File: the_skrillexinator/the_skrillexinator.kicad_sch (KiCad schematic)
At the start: 0 parts

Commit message: add shit
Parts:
- added J1, J2: Conn_01x03, symbol Connector_Generic:Conn_01x03
- added U1: ESP32-WROOM-32, RF_Module:ESP32-WROOM-32, symbol RF_Module:ESP32-WROOM-32
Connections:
- new net: J2.2 (Pin_2), U1.36 (IO22)
- new net +3.3V: J2.3 (Pin_3), U1.2 (VDD)
- new net GND: J2.1 (Pin_1), U1.1 (GND), U1.15 (GND), U1.38 (GND), U1.39 (GND)

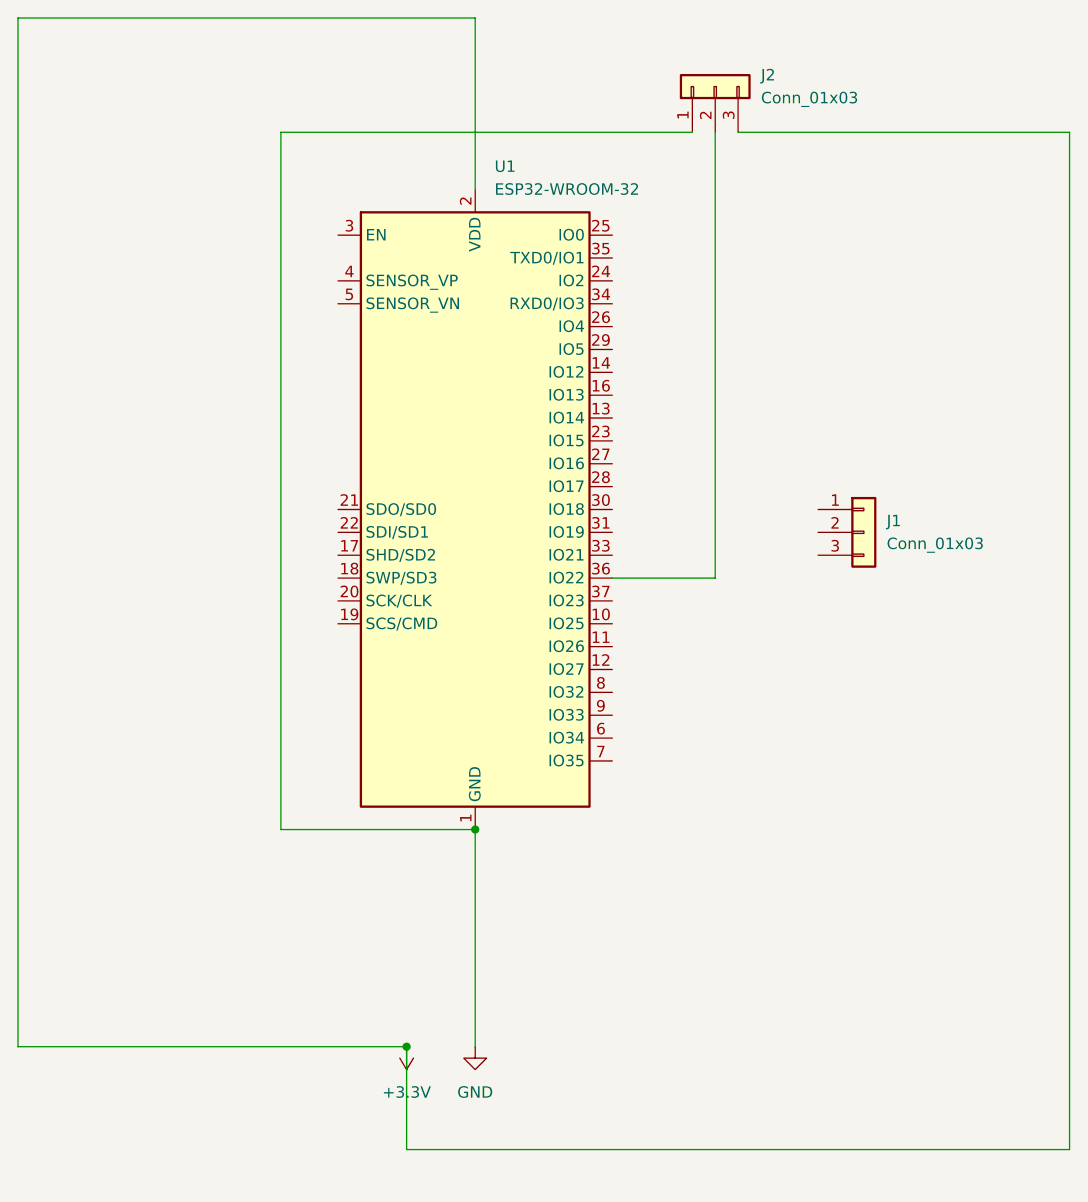
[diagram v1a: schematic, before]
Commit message: add resistor shit
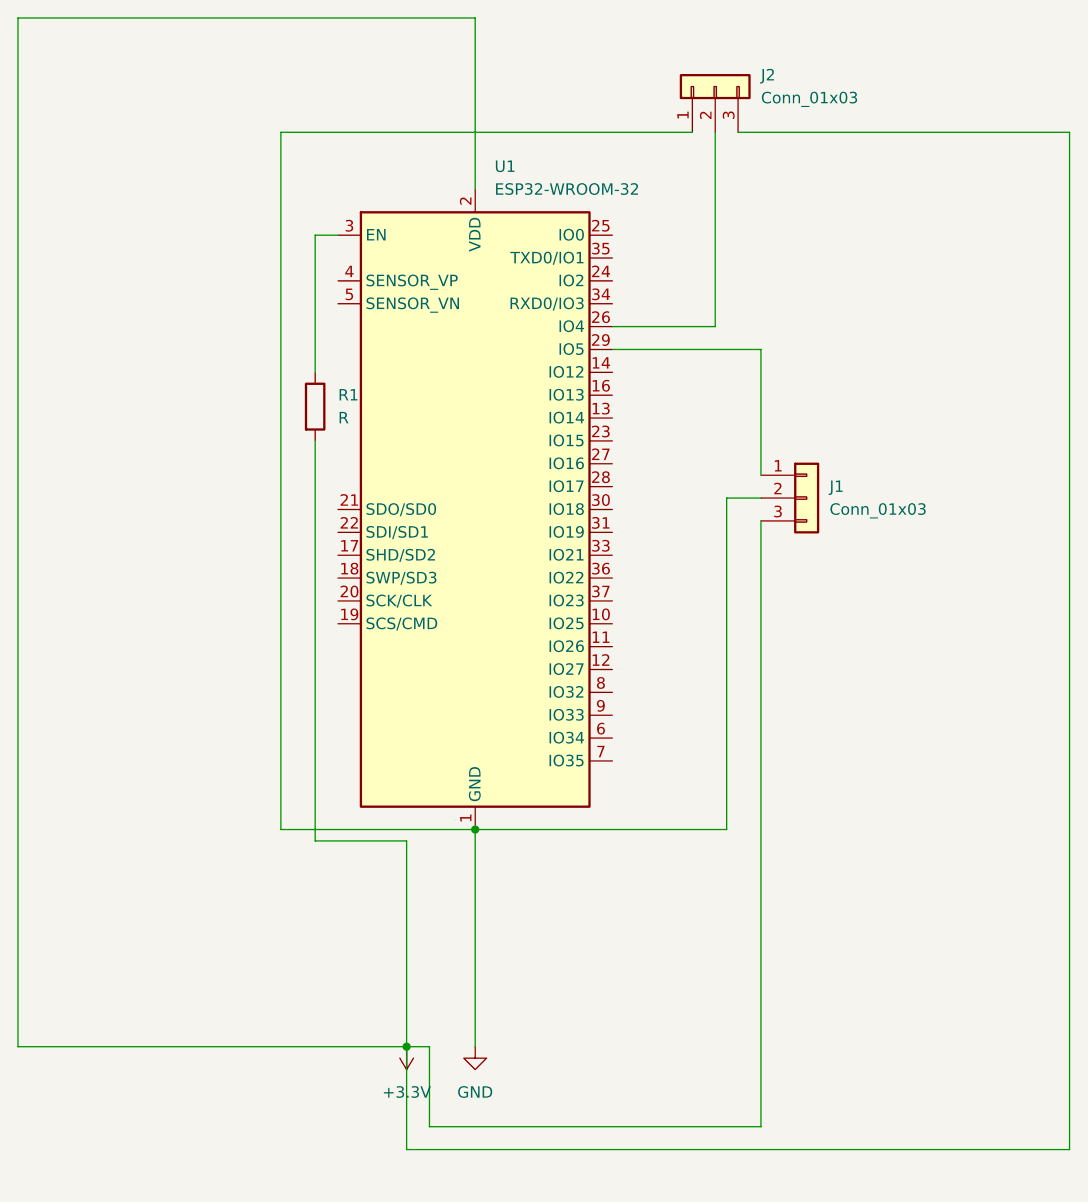
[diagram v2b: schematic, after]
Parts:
- added R1: R, symbol Device:R
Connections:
- net +3.3V: now also J1.3 (Pin_3), R1.2
- net GND: now also J1.2 (Pin_2)
- net at U1.26 (IO4): now also J2.2 (Pin_2)
- net at U1.29 (IO5): now also J1.1 (Pin_1)
- net at U1.3 (EN): now also R1.1
- net at U1.36 (IO22): no longer J2.2 (Pin_2)
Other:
- moved on the sheet: J1
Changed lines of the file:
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@@
+	(wire
+		(pts
+			(xy 181.61 76.2) (xy 181.61 62.23)
+		)
+		(stroke
+			(width 0)
+			(type default)
+		)
+	)
 	(wire
 		(pts
@@
 	(wire
 		(pts
+			(xy 132.08 116.84) (xy 142.24 116.84)
+		)
+		(stroke
+			(width 0)
+			(type default)
+		)
+	)
+	(wire
+		(pts
+			(xy 176.53 59.69) (xy 165.1 59.69)
+		)
+		(stroke
+			(width 0)
+			(type default)
+		)
+	)
+	(wire
+		(pts
+			(xy 132.08 64.77) (xy 132.08 49.53)
+		)
+		(stroke
+			(width 0)
+			(type default)
+		)
+	)
+	(wire
+		(pts
 			(xy 149.86 25.4) (xy 99.06 25.4)
 		)
@@
 	(wire
 		(pts
+			(xy 144.78 148.59) (xy 144.78 139.7)
+		)
+		(stroke
+			(width 0)
+			(type default)
+		)
+	)
+	(wire
+		(pts
+			(xy 181.61 78.74) (xy 177.8 78.74)
+		)
+		(stroke
+			(width 0)
+			(type default)
+		)
+	)
+	(wire
+		(pts
 			(xy 215.9 38.1) (xy 215.9 151.13)
 		)
@@
 	(wire
 		(pts
+			(xy 142.24 116.84) (xy 142.24 139.7)
+		)
+		(stroke
+			(width 0)
+			(type default)
+		)
+	)
+	(wire
+		(pts
 			(xy 128.27 115.57) (xy 149.86 115.57)
 		)
@@
 	(wire
 		(pts
-			(xy 165.1 87.63) (xy 176.53 87.63)
+			(xy 181.61 62.23) (xy 165.1 62.23)
+		)
+		(stroke
+			(width 0)
+			(type default)
+		)
+	)
+	(wire
+		(pts
+			(xy 176.53 38.1) (xy 176.53 59.69)
 		)
 		(stroke
@@
 	(wire
 		(pts
-			(xy 176.53 87.63) (xy 176.53 38.1)
+			(xy 132.08 49.53) (xy 134.62 49.53)
+		)
+		(stroke
+			(width 0)
+			(type default)
+		)
+	)
+	(wire
+		(pts
+			(xy 132.08 72.39) (xy 132.08 116.84)
 		)
 		(stroke
@@
 	(wire
 		(pts
+			(xy 177.8 78.74) (xy 177.8 115.57)
+		)
+		(stroke
+			(width 0)
+			(type default)
+		)
+	)
+	(wire
+		(pts
 			(xy 149.86 44.45) (xy 149.86 25.4)
 		)
@@
 	(wire
 		(pts
+			(xy 177.8 115.57) (xy 149.86 115.57)
+		)
+		(stroke
+			(width 0)
+			(type default)
+		)
+	)
+	(wire
+		(pts
+			(xy 181.61 148.59) (xy 144.78 148.59)
+		)
+		(stroke
+			(width 0)
+			(type default)
+		)
+	)
+	(wire
+		(pts
 			(xy 99.06 139.7) (xy 142.24 139.7)
 		)
@@
 	(wire
 		(pts
+			(xy 181.61 81.28) (xy 181.61 148.59)
+		)
+		(stroke
+			(width 0)
+			(type default)
+		)
+	)
+	(wire
+		(pts
+			(xy 144.78 139.7) (xy 142.24 139.7)
+		)
+		(stroke
+			(width 0)
+			(type default)
+		)
+	)
+	(wire
+		(pts
 			(xy 215.9 151.13) (xy 142.24 151.13)
 		)
@@
 			(width 0)
 			(type default)
+		)
+	)
+	(symbol
+		(lib_id "Device:R")
+		(at 132.08 68.58 0)
+		(unit 1)
+		(body_style 1)
+		(exclude_from_sim no)
+		(in_bom yes)
+		(on_board yes)
+		(in_pos_files yes)
+		(dnp no)
+		(fields_autoplaced yes)
+		(property "Reference" "R1"
+			(at 134.62 67.3099 0)
+			(show_name no)
+			(do_not_autoplace no)
+			(effects
+				(font
+					(size 1.27 1.27)
+				)
+				(justify left)
+			)
+		)
+		(property "Value" "R"
+			(at 134.62 69.8499 0)
+			(show_name no)
+			(do_not_autoplace no)
+			(effects
+				(font
+					(size 1.27 1.27)
+				)
+				(justify left)
+			)
+		)
+		(property "Footprint" ""
+			(at 130.302 68.58 90)
+			(hide yes)
+			(show_name no)
+			(do_not_autoplace no)
+			(effects
+				(font
+					(size 1.27 1.27)
+				)
+			)
+		)
+		(property "Datasheet" ""
+			(at 132.08 68.58 0)
+			(hide yes)
+			(show_name no)
+			(do_not_autoplace no)
+			(effects
+				(font
+					(size 1.27 1.27)
+				)
+			)
+		)
+		(property "Description" "Resistor"
+			(at 132.08 68.58 0)
+			(hide yes)
+			(show_name no)
+			(do_not_autoplace no)
+			(effects
+				(font
+					(size 1.27 1.27)
+				)
+			)
+		)
+		(pin "1"
+		)
+		(pin "2"
+		)
+		(instances
+			(project "the_skrillexinator"
+				(path "/76fe25bb-3898-44a0-a654-1d7be38cc137"
+					(reference "R1")
+					(unit 1)
+				)
+			)
 		)
 	)
@@
 	(symbol
 		(lib_id "Connector_Generic:Conn_01x03")
-		(at 193.04 82.55 0)
+		(at 186.69 78.74 0)
 		(unit 1)
 		(body_style 1)
@@
 		(fields_autoplaced yes)
 		(property "Reference" "J1"
-			(at 195.58 81.2799 0)
+			(at 189.23 77.4699 0)
 			(show_name no)
 			(do_not_autoplace no)
@@
 		)
 		(property "Value" "Conn_01x03"
-			(at 195.58 83.8199 0)
+			(at 189.23 80.0099 0)
 			(show_name no)
 			(do_not_autoplace no)
@@
 		)
 		(property "Footprint" ""
-			(at 193.04 82.55 0)
+			(at 186.69 78.74 0)
 			(hide yes)
 			(show_name no)
@@
 		)
 		(property "Datasheet" ""
-			(at 193.04 82.55 0)
+			(at 186.69 78.74 0)
 			(hide yes)
 			(show_name no)
@@
 		)
 		(property "Description" "Generic connector, single row, 01x03, script generated (kicad-library-utils/schlib/autogen/connector/)"
-			(at 193.04 82.55 0)
-			(hide yes)
-			(show_name no)
+			(at 186.69 78.74 0)
+			(hide yes)
+			(show_name no)

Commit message: add resistor shit
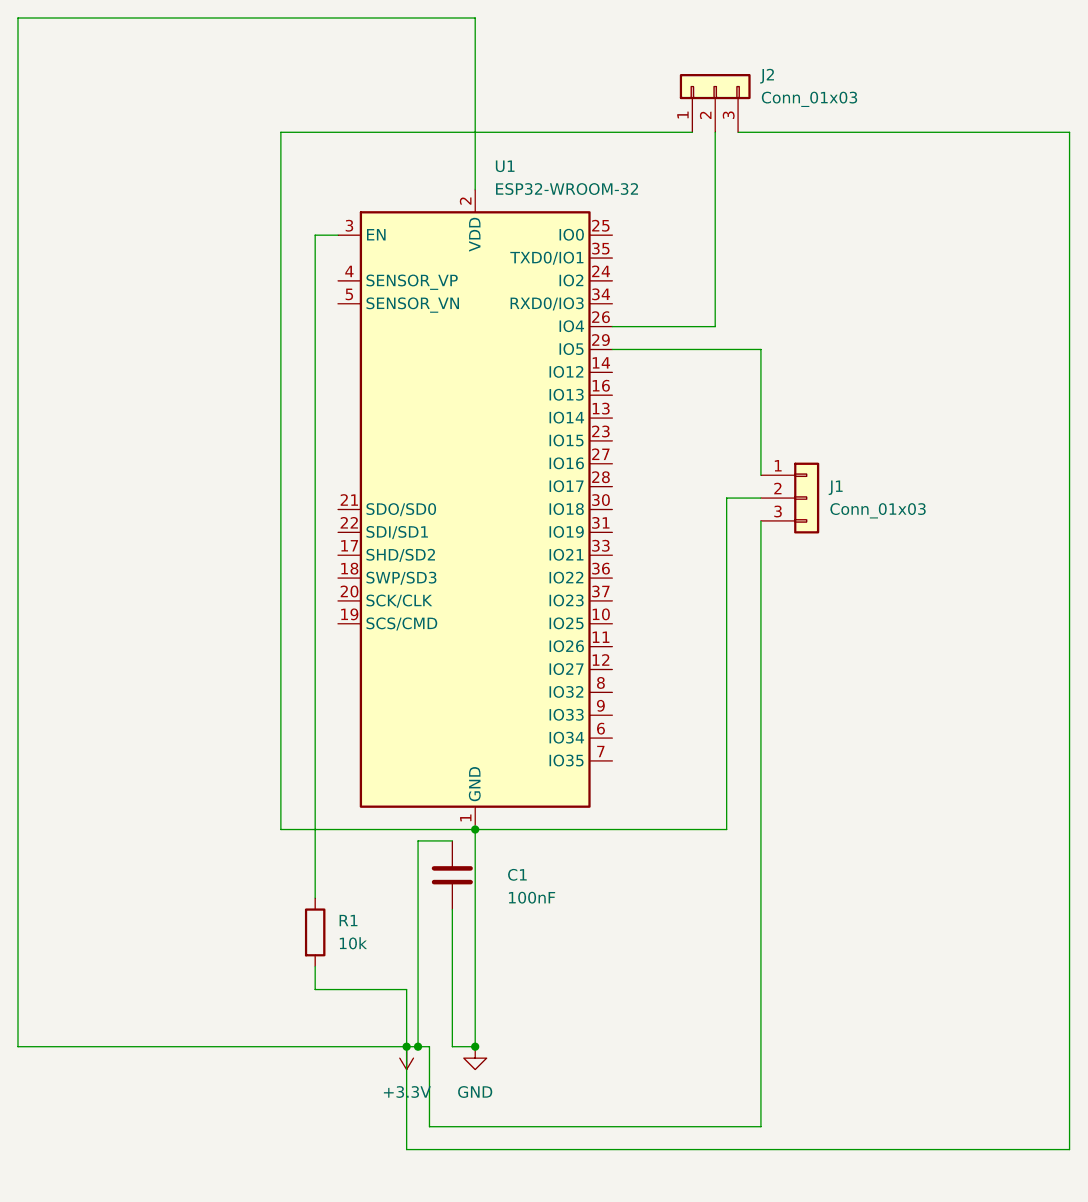
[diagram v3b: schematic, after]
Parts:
- added C1: 100nF, symbol Device:C
- R1: value R -> 10k
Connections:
- net +3.3V: now also C1.1
- net GND: now also C1.2
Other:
- moved on the sheet: R1
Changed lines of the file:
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@@
 	(paper "A4")
+	(junction
+		(at 143.51 139.7)
+		(diameter 0)
+		(color 0 0 0 0)
+	)
+	(junction
+		(at 149.86 139.7)
+		(diameter 0)
+		(color 0 0 0 0)
+	)
 	(junction
 		(at 142.24 139.7)
@@
 	(wire
 		(pts
+			(xy 143.51 139.7) (xy 144.78 139.7)
+		)
+		(stroke
+			(width 0)
+			(type default)
+		)
+	)
+	(wire
+		(pts
 			(xy 142.24 151.13) (xy 142.24 139.7)
 		)
@@
 	(wire
 		(pts
-			(xy 132.08 116.84) (xy 142.24 116.84)
+			(xy 132.08 133.35) (xy 142.24 133.35)
 		)
 		(stroke
@@
 	(wire
 		(pts
-			(xy 132.08 64.77) (xy 132.08 49.53)
+			(xy 132.08 123.19) (xy 132.08 49.53)
 		)
 		(stroke
@@
 	(wire
 		(pts
-			(xy 142.24 116.84) (xy 142.24 139.7)
+			(xy 142.24 133.35) (xy 142.24 139.7)
 		)
 		(stroke
@@
 	(wire
 		(pts
+			(xy 147.32 139.7) (xy 149.86 139.7)
+		)
+		(stroke
+			(width 0)
+			(type default)
+		)
+	)
+	(wire
+		(pts
 			(xy 181.61 62.23) (xy 165.1 62.23)
 		)
@@
 	(wire
 		(pts
+			(xy 147.32 124.46) (xy 147.32 139.7)
+		)
+		(stroke
+			(width 0)
+			(type default)
+		)
+	)
+	(wire
+		(pts
+			(xy 143.51 139.7) (xy 143.51 116.84)
+		)
+		(stroke
+			(width 0)
+			(type default)
+		)
+	)
+	(wire
+		(pts
 			(xy 128.27 38.1) (xy 128.27 115.57)
 		)
@@
 	(wire
 		(pts
-			(xy 132.08 72.39) (xy 132.08 116.84)
+			(xy 132.08 130.81) (xy 132.08 133.35)
 		)
 		(stroke
@@
 	(wire
 		(pts
-			(xy 144.78 139.7) (xy 142.24 139.7)
+			(xy 143.51 116.84) (xy 147.32 116.84)
+		)
+		(stroke
+			(width 0)
+			(type default)
+		)
+	)
+	(wire
+		(pts
+			(xy 142.24 139.7) (xy 143.51 139.7)
 		)
 		(stroke
@@
 	(symbol
 		(lib_id "Device:R")
-		(at 132.08 68.58 0)
+		(at 132.08 127 0)
 		(unit 1)
 		(body_style 1)
@@
 		(fields_autoplaced yes)
 		(property "Reference" "R1"
-			(at 134.62 67.3099 0)
+			(at 134.62 125.7299 0)
 			(show_name no)
 			(do_not_autoplace no)
@@
 			)
 		)
-		(property "Value" "R"
-			(at 134.62 69.8499 0)
+		(property "Value" "10k"
+			(at 134.62 128.2699 0)
 			(show_name no)
 			(do_not_autoplace no)
@@
 		)
 		(property "Footprint" ""
-			(at 130.302 68.58 90)
+			(at 130.302 127 90)
 			(hide yes)
 			(show_name no)
@@
 		)
 		(property "Datasheet" ""
-			(at 132.08 68.58 0)
+			(at 132.08 127 0)
 			(hide yes)
 			(show_name no)
@@
 		)
 		(property "Description" "Resistor"
-			(at 132.08 68.58 0)
+			(at 132.08 127 0)
 			(hide yes)
 			(show_name no)
@@
 					(unit 1)
 				)
+			)
+		)
+	)
+	(symbol
+		(lib_id "Device:C")
+		(at 147.32 120.65 0)
+		(unit 1)
+		(body_style 1)
+		(exclude_from_sim no)
+		(in_bom yes)
+		(on_board yes)
+		(in_pos_files yes)
+		(dnp no)
+		(property "Reference" "C1"
+			(at 153.416 120.65 0)
+			(show_name no)
+			(do_not_autoplace no)
+			(effects
+				(font
+					(size 1.27 1.27)
+				)
+				(justify left)
+			)
+		)
+		(property "Value" "100nF"
+			(at 153.416 123.19 0)
+			(show_name no)
+			(do_not_autoplace no)
+			(effects
+				(font
+					(size 1.27 1.27)
+				)
+				(justify left)
+			)
+		)
+		(property "Footprint" ""
+			(at 148.2852 124.46 0)
+			(hide yes)
+			(show_name no)
+			(do_not_autoplace no)
+			(effects
+				(font
+					(size 1.27 1.27)
+				)
+			)
+		)
+		(property "Datasheet" ""
+			(at 147.32 120.65 0)
+			(hide yes)
+			(show_name no)
+			(do_not_autoplace no)
+			(effects
+				(font
+					(size 1.27 1.27)
+				)
+			)
+		)
+		(property "Description" "Unpolarized capacitor"
+			(at 147.32 120.65 0)
+			(hide yes)
+			(show_name no)
+			(do_not_autoplace no)
+			(effects
+				(font
+					(size 1.27 1.27)
+				)
+			)
+		)
+		(pin "2"
+		)
+		(pin "1"
+		)
+		(instances
+			(project "the_skrillexinator"
+				(path "/76fe25bb-3898-44a0-a654-1d7be38cc137"
+					(reference "C1")
+					(unit 1)
+				)

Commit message: add di powa
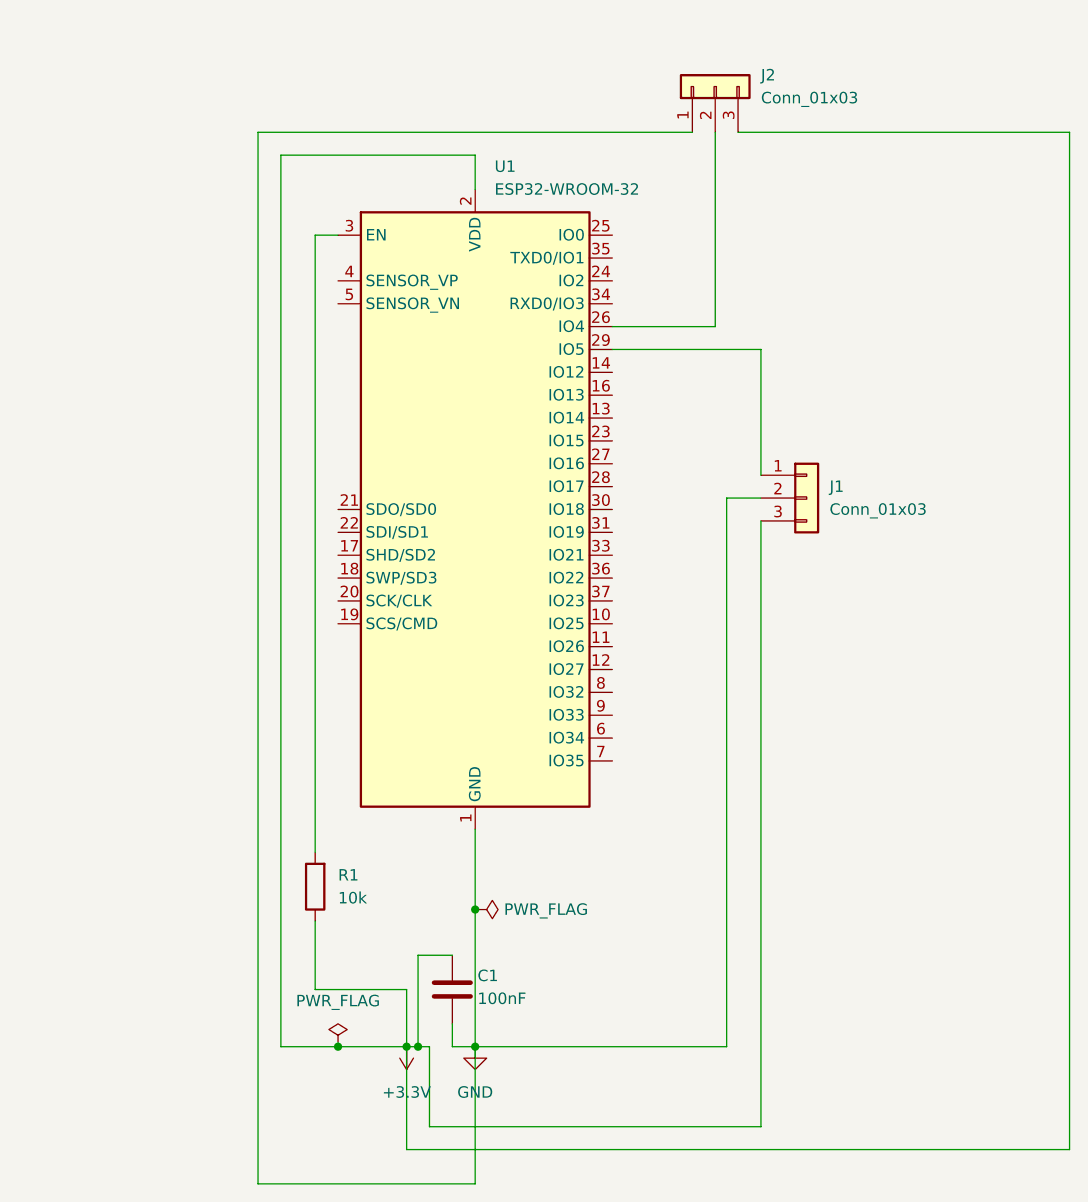
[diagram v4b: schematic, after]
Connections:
- net +3.3V: now also R1.1; no longer R1.2
- net at U1.3 (EN): now also R1.2; no longer R1.1
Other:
- moved on the sheet: C1, R1
